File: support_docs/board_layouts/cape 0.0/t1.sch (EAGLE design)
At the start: 14 parts, among them IC1 74HC595N

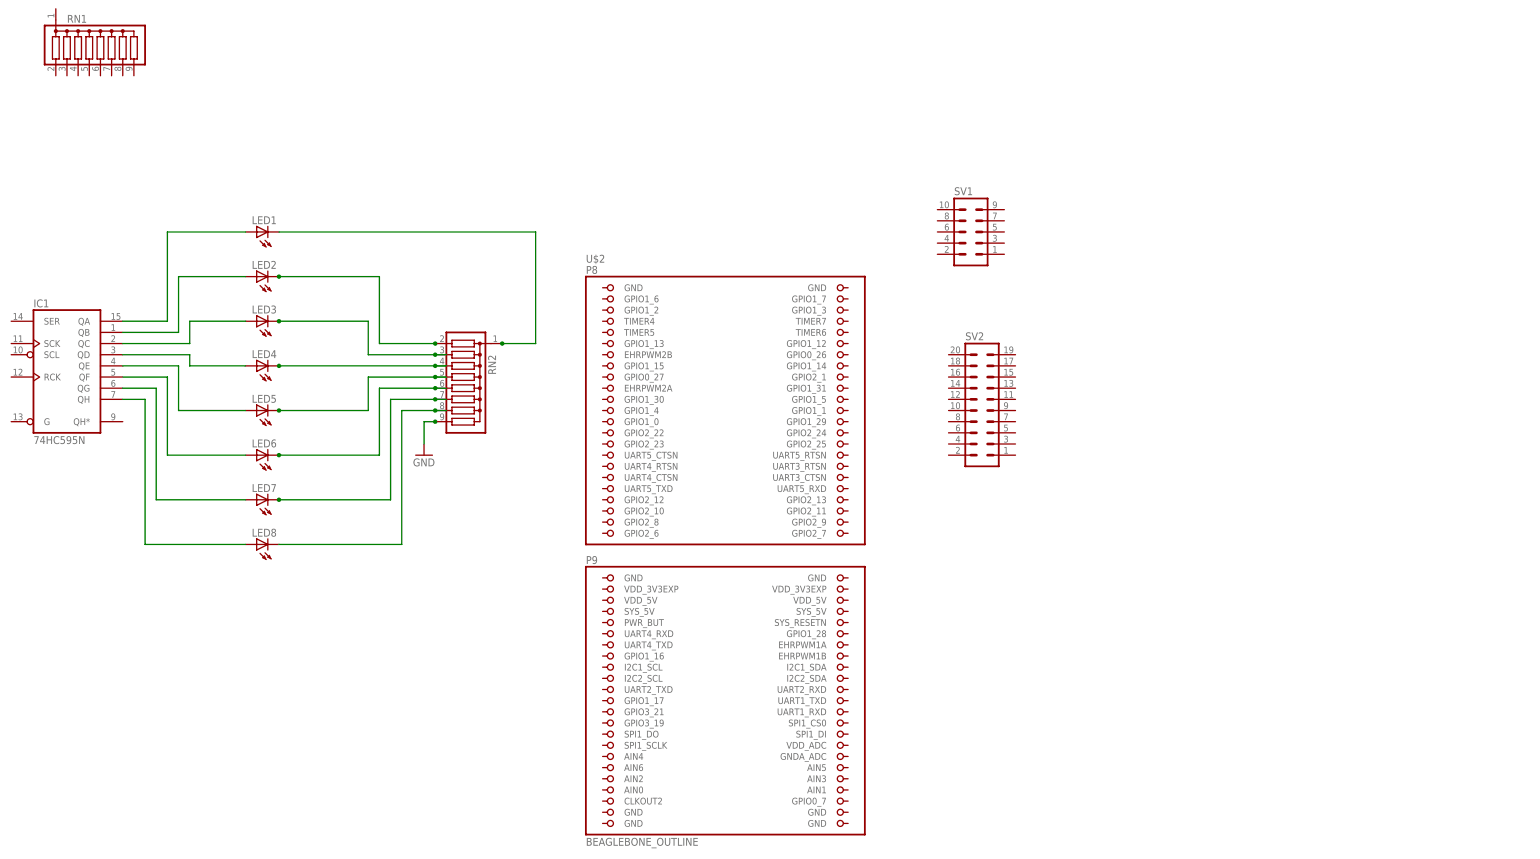
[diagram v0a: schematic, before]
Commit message: testing and updating cape layout
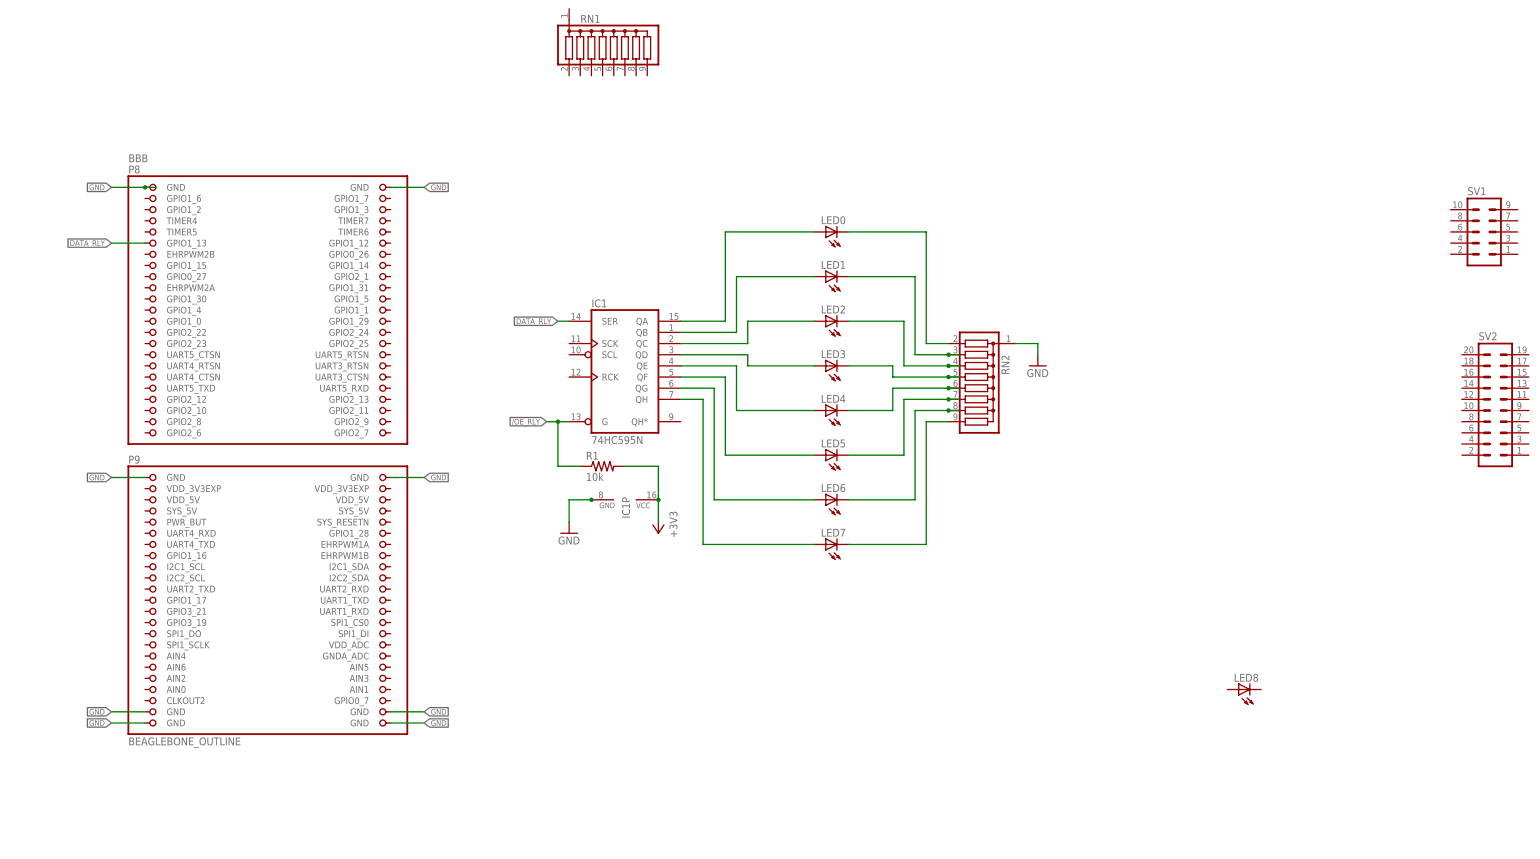
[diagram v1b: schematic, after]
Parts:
- removed U$2: BEAGLEBONE_OUTLINE, local:BEAGLEBONE_OUTLINE
- added BBB: BEAGLEBONE_OUTLINE, local:BEAGLEBONE_OUTLINE
- added LED0: (no value), adafruit:LED3MM
- added R1: 10k, rcl:R-US_0207/12
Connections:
- removed net N$1: LED1.C, RN2.1
- new net +3V3: IC1P.VCC, R1.2
- new net /OE_RLY: IC1A.G, R1.1
- new net DATA_RLY: BBB.GPIO1_13, IC1A.SER
- new net N$17: IC1A.QH, LED7.A
- net GND: now also BBB.GND@1, BBB.GND@2, BBB.GND@3, BBB.GND@4, BBB.GND@5, BBB.GND@6, BBB.GND@7, BBB.GND@8, IC1P.GND, RN2.1; no longer RN2.9
- net N$10: now also LED5.C, RN2.7; no longer IC1A.QB, LED2.A
- net N$11: now also LED2.A; no longer LED3.A
- net N$12: now also LED3.A; no longer LED4.A
- net N$13: now also LED4.A; no longer LED5.A
- net N$14: now also LED5.A; no longer LED6.A
- net N$15: now also LED7.C, RN2.9; no longer IC1A.QG, LED7.A
- net N$16: now also IC1A.QG, LED6.A; no longer IC1A.QH, LED8.A
- net N$2: now also LED1.C, RN2.3; no longer LED2.C, RN2.2
- net N$3: now also RN2.5; no longer RN2.3
- net N$4: now also LED2.C; no longer LED4.C
- net N$5: now also LED4.C, RN2.6; no longer LED5.C, RN2.5
- net N$6: now also RN2.8; no longer RN2.6
- net N$7: now also LED0.C, RN2.2; no longer LED7.C, RN2.7
- net N$8: now also IC1A.QA, LED0.A; no longer LED8.C, RN2.8
- net N$9: now also IC1A.QB; no longer IC1A.QA
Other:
- moved on the sheet: IC1, LED1, LED2, LED3, LED4, LED5, LED6, LED7, LED8, RN1, RN2, SV1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
